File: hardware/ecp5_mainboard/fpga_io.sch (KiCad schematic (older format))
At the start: 75 parts, among them J10 UART, J11 FLASH, J12 JTAG, J5 EXT0, J6 EXT1, J7 EXT2, J8 EXT3, J9 PMOD_01, Q9 BSH111BKR, SW6 SW_Push, U15 ECP5UM5G_85_CABGA756, U26 XL_XO_LVDS, U27 W25Q

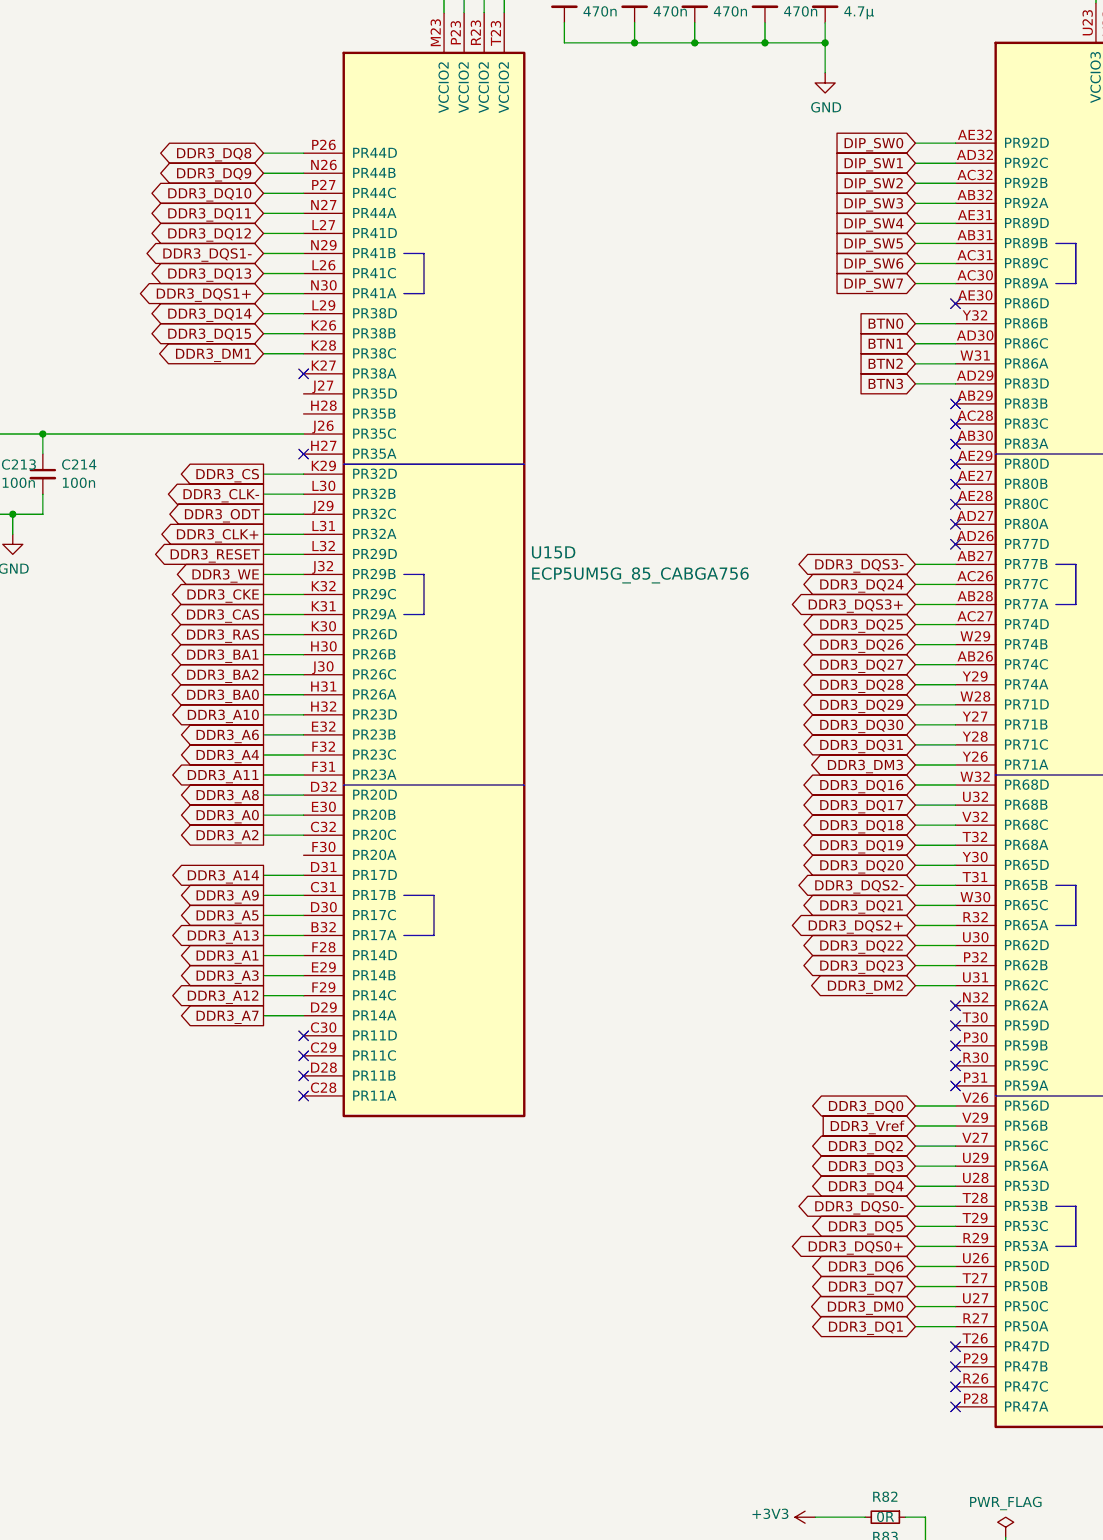
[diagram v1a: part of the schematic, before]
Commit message: hardware/mainboard: Route DDR3 bytes 0 and 1
Signed-off-by: David Shah <dave@ds0.me>
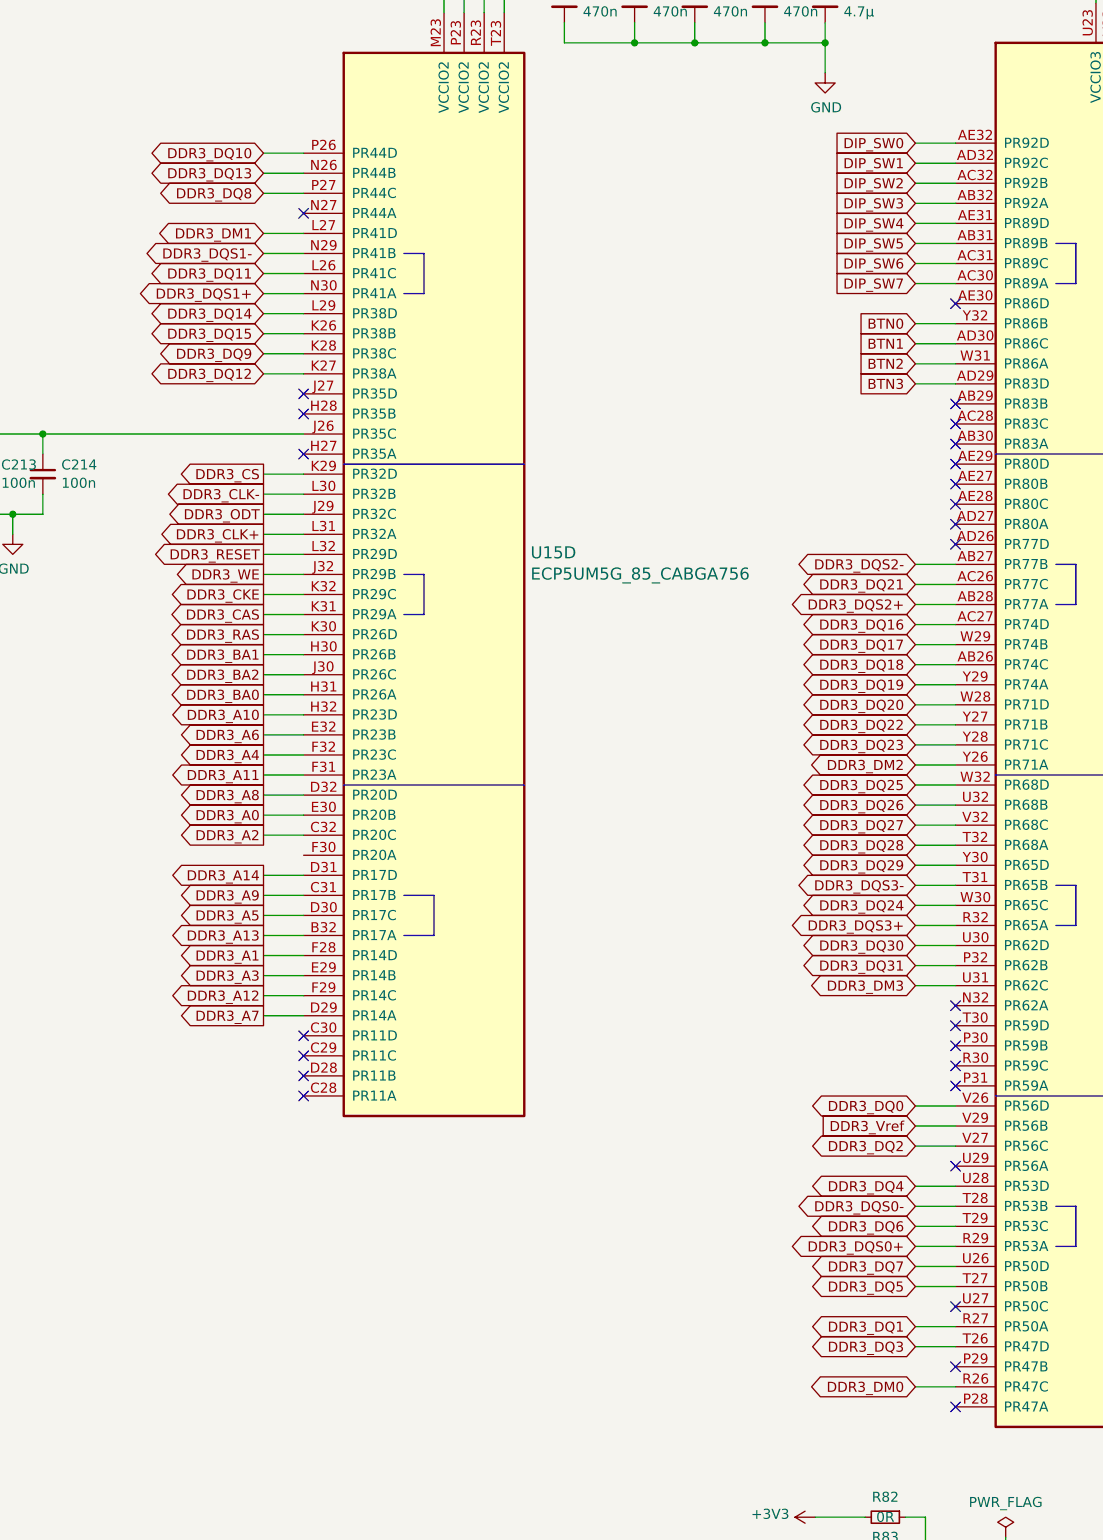
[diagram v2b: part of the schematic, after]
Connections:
- net DDR3_DM0: now also U15.R26 (PR47C); no longer U15.U27 (PR50C)
- net DDR3_DM1: now also U15.L27 (PR41D); no longer U15.K28 (PR38C)
- net DDR3_DM2: now also U15.Y26 (PR71A); no longer U15.U31 (PR62C)
- net DDR3_DM3: now also U15.U31 (PR62C); no longer U15.Y26 (PR71A)
- net DDR3_DQ10: now also U15.P26 (PR44D); no longer U15.P27 (PR44C)
- net DDR3_DQ11: now also U15.L26 (PR41C); no longer U15.N27 (PR44A)
- net DDR3_DQ12: now also U15.K27 (PR38A); no longer U15.L27 (PR41D)
- net DDR3_DQ13: now also U15.N26 (PR44B); no longer U15.L26 (PR41C)
- net DDR3_DQ16: now also U15.AC27 (PR74D); no longer U15.W32 (PR68D)
- net DDR3_DQ17: now also U15.W29 (PR74B); no longer U15.U32 (PR68B)
- net DDR3_DQ18: now also U15.AB26 (PR74C); no longer U15.V32 (PR68C)
- net DDR3_DQ19: now also U15.Y29 (PR74A); no longer U15.T32 (PR68A)
- net DDR3_DQ20: now also U15.W28 (PR71D); no longer U15.Y30 (PR65D)
- net DDR3_DQ21: now also U15.AC26 (PR77C); no longer U15.W30 (PR65C)
- net DDR3_DQ22: now also U15.Y27 (PR71B); no longer U15.U30 (PR62D)
- net DDR3_DQ23: now also U15.Y28 (PR71C); no longer U15.P32 (PR62B)
- net DDR3_DQ24: now also U15.W30 (PR65C); no longer U15.AC26 (PR77C)
- net DDR3_DQ25: now also U15.W32 (PR68D); no longer U15.AC27 (PR74D)
- net DDR3_DQ26: now also U15.U32 (PR68B); no longer U15.W29 (PR74B)
- net DDR3_DQ27: now also U15.V32 (PR68C); no longer U15.AB26 (PR74C)
- net DDR3_DQ28: now also U15.T32 (PR68A); no longer U15.Y29 (PR74A)
- net DDR3_DQ29: now also U15.Y30 (PR65D); no longer U15.W28 (PR71D)
- net DDR3_DQ3: now also U15.T26 (PR47D); no longer U15.U29 (PR56A)
- net DDR3_DQ30: now also U15.U30 (PR62D); no longer U15.Y27 (PR71B)
- net DDR3_DQ31: now also U15.P32 (PR62B); no longer U15.Y28 (PR71C)
- net DDR3_DQ5: now also U15.T27 (PR50B); no longer U15.T29 (PR53C)
- net DDR3_DQ6: now also U15.T29 (PR53C); no longer U15.U26 (PR50D)
- net DDR3_DQ7: now also U15.U26 (PR50D); no longer U15.T27 (PR50B)
- net DDR3_DQ8: now also U15.P27 (PR44C); no longer U15.P26 (PR44D)
- net DDR3_DQ9: now also U15.K28 (PR38C); no longer U15.N26 (PR44B)
- net DDR3_DQS2+: now also U15.AB28 (PR77A); no longer U15.R32 (PR65A)
- net DDR3_DQS2-: now also U15.AB27 (PR77B); no longer U15.T31 (PR65B)
- net DDR3_DQS3+: now also U15.R32 (PR65A); no longer U15.AB28 (PR77A)
- net DDR3_DQS3-: now also U15.T31 (PR65B); no longer U15.AB27 (PR77B)
- no-connect marks 61 -> 63
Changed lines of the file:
@@
 Text GLabel 2150 2450 0    50   BiDi ~ 0
 DDR3_DQS1-
-Text GLabel 2150 1950 0    50   BiDi ~ 0
+Text GLabel 2150 2150 0    50   BiDi ~ 0
 DDR3_DQ8
-Text GLabel 2150 2050 0    50   BiDi ~ 0
+Text GLabel 2150 2950 0    50   BiDi ~ 0
 DDR3_DQ9
-Text GLabel 2150 2150 0    50   BiDi ~ 0
+Text GLabel 2150 1950 0    50   BiDi ~ 0
 DDR3_DQ10
-Text GLabel 2150 2250 0    50   BiDi ~ 0
+Text GLabel 2150 2550 0    50   BiDi ~ 0
 DDR3_DQ11
-Text GLabel 2150 2350 0    50   BiDi ~ 0
+Text GLabel 2150 3050 0    50   BiDi ~ 0
 DDR3_DQ12
-Text GLabel 2150 2550 0    50   BiDi ~ 0
+Text GLabel 2150 2050 0    50   BiDi ~ 0
 DDR3_DQ13
 Text GLabel 2150 2750 0    50   BiDi ~ 0
@@
 Text GLabel 2150 2850 0    50   BiDi ~ 0
 DDR3_DQ15
-Text GLabel 2150 2950 0    50   BiDi ~ 0
+Text GLabel 2150 2350 0    50   BiDi ~ 0
 DDR3_DM1
 Wire Wire Line
-	2150 1950 2350 1950
+	2150 2150 2350 2150
 Wire Wire Line
-	2150 2050 2350 2050
+	2150 2950 2350 2950
 Wire Wire Line
-	2150 2150 2350 2150
+	2150 1950 2350 1950
 Wire Wire Line
-	2150 2250 2350 2250
+	2150 2550 2350 2550
 Wire Wire Line
-	2150 2350 2350 2350
+	2150 3050 2350 3050
 Wire Wire Line
 	2150 2450 2350 2450
 Wire Wire Line
-	2150 2550 2350 2550
+	2150 2050 2350 2050
 Wire Wire Line
 	2150 2650 2350 2650
@@
 	2150 2850 2350 2850
 Wire Wire Line
-	2150 2950 2350 2950
+	2150 2350 2350 2350
 Wire Wire Line
 	15400 1800 14800 1800
@@
 Text Label 14800 2000 0    50   ~ 0
 CLK100+
-Text GLabel 5400 5800 0    50   BiDi ~ 0
+Text GLabel 5400 4200 0    50   BiDi ~ 0
 DDR3_DQS2+
-Text GLabel 5400 5600 0    50   BiDi ~ 0
+Text GLabel 5400 4000 0    50   BiDi ~ 0
 DDR3_DQS2-
-Text GLabel 5400 5100 0    50   BiDi ~ 0
+Text GLabel 5400 4300 0    50   BiDi ~ 0
 DDR3_DQ16
-Text GLabel 5400 5200 0    50   BiDi ~ 0
+Text GLabel 5400 4400 0    50   BiDi ~ 0
 DDR3_DQ17
-Text GLabel 5400 5300 0    50   BiDi ~ 0
+Text GLabel 5400 4500 0    50   BiDi ~ 0
 DDR3_DQ18
-Text GLabel 5400 5400 0    50   BiDi ~ 0
+Text GLabel 5400 4600 0    50   BiDi ~ 0
 DDR3_DQ19
-Text GLabel 5400 5500 0    50   BiDi ~ 0
+Text GLabel 5400 4700 0    50   BiDi ~ 0
 DDR3_DQ20
-Text GLabel 5400 5700 0    50   BiDi ~ 0
+Text GLabel 5400 4100 0    50   BiDi ~ 0
 DDR3_DQ21
-Text GLabel 5400 5900 0    50   BiDi ~ 0
+Text GLabel 5400 4800 0    50   BiDi ~ 0
 DDR3_DQ22
-Text GLabel 5400 6000 0    50   BiDi ~ 0
+Text GLabel 5400 4900 0    50   BiDi ~ 0
 DDR3_DQ23
 Wire Wire Line
-	5400 5100 5600 5100
+	5400 4300 5600 4300
 Wire Wire Line
-	5400 5200 5600 5200
+	5400 4400 5600 4400
 Wire Wire Line
-	5400 5300 5600 5300
+	5400 4500 5600 4500
 Wire Wire Line
-	5400 5400 5600 5400
+	5400 4600 5600 4600
 Wire Wire Line
-	5400 5500 5600 5500
+	5400 4700 5600 4700
 Wire Wire Line
-	5400 5600 5600 5600
+	5400 4000 5600 4000
 Wire Wire Line
-	5400 5700 5600 5700
+	5400 4100 5600 4100
 Wire Wire Line
-	5400 5800 5600 5800
+	5400 4200 5600 4200
 Wire Wire Line
-	5400 5900 5600 5900
+	5400 4800 5600 4800
 Wire Wire Line
-	5400 6000 5600 6000
-Text GLabel 5400 6100 0    50   BiDi ~ 0
+	5400 4900 5600 4900
+Text GLabel 5400 5000 0    50   BiDi ~ 0
 DDR3_DM2
 Wire Wire Line
-	5400 6100 5600 6100
+	5400 5000 5600 5000
 $Comp
 L Device:C_Small C218
@@
 Wire Wire Line
 	5400 6800 5600 6800
-Text GLabel 5400 4200 0    50   BiDi ~ 0
+Text GLabel 5400 5800 0    50   BiDi ~ 0
 DDR3_DQS3+
 Wire Wire Line
-	5400 4200 5600 4200
-Text GLabel 5400 4000 0    50   BiDi ~ 0
+	5400 5800 5600 5800
+Text GLabel 5400 5600 0    50   BiDi ~ 0
 DDR3_DQS3-
 Wire Wire Line
-	5400 4000 5600 4000
+	5400 5600 5600 5600
 Wire Wire Line
-	5600 4100 5400 4100
-Text GLabel 5400 4100 0    50   BiDi ~ 0
+	5600 5700 5400 5700
+Text GLabel 5400 5700 0    50   BiDi ~ 0
 DDR3_DQ24
-Text GLabel 5400 4300 0    50   BiDi ~ 0
+Text GLabel 5400 5100 0    50   BiDi ~ 0
 DDR3_DQ25
-Text GLabel 5400 4400 0    50   BiDi ~ 0
+Text GLabel 5400 5200 0    50   BiDi ~ 0
 DDR3_DQ26
-Text GLabel 5400 4500 0    50   BiDi ~ 0
+Text GLabel 5400 5300 0    50   BiDi ~ 0
 DDR3_DQ27
-Text GLabel 5400 4600 0    50   BiDi ~ 0
+Text GLabel 5400 5400 0    50   BiDi ~ 0
 DDR3_DQ28
-Text GLabel 5400 4700 0    50   BiDi ~ 0
+Text GLabel 5400 5500 0    50   BiDi ~ 0
 DDR3_DQ29
-Text GLabel 5400 4800 0    50   BiDi ~ 0
+Text GLabel 5400 5900 0    50   BiDi ~ 0
 DDR3_DQ30
-Text GLabel 5400 4900 0    50   BiDi ~ 0
+Text GLabel 5400 6000 0    50   BiDi ~ 0
 DDR3_DQ31
 Wire Wire Line
-	5400 4900 5600 4900
+	5400 6000 5600 6000
 Wire Wire Line
-	5600 4800 5400 4800
+	5600 5900 5400 5900
 Wire Wire Line
-	5400 4700 5600 4700
+	5400 5500 5600 5500
 Wire Wire Line
-	5600 4600 5400 4600
+	5600 5400 5400 5400
 Wire Wire Line
-	5400 4500 5600 4500
+	5400 5300 5600 5300
 Wire Wire Line
-	5600 4400 5400 4400
+	5600 5200 5400 5200
 Wire Wire Line
-	5400 4300 5600 4300
+	5400 5100 5600 5100
 Text GLabel 2150 5250 0    50   Output ~ 0
 DDR3_A0
@@
 Text GLabel 2150 3550 0    50   Output ~ 0
 DDR3_CS
-Text GLabel 5400 5000 0    50   BiDi ~ 0
+Text GLabel 5400 6100 0    50   BiDi ~ 0
 DDR3_DM3
 Wire Wire Line
-	5400 5000 5600 5000
+	5400 6100 5600 6100
 Wire Wire Line
 	2150 3950 2350 3950
@@
 Text GLabel 5400 6900 0    50   BiDi ~ 0
 DDR3_DQ2
-Text GLabel 5400 7000 0    50   BiDi ~ 0
+Text GLabel 5400 7900 0    50   BiDi ~ 0
 DDR3_DQ3
 Text GLabel 5400 7100 0    50   BiDi ~ 0
 DDR3_DQ4
-Text GLabel 5400 7300 0    50   BiDi ~ 0
+Text GLabel 5400 7600 0    50   BiDi ~ 0
 DDR3_DQ5
-Text GLabel 5400 7500 0    50   BiDi ~ 0
+Text GLabel 5400 7300 0    50   BiDi ~ 0
 DDR3_DQ6
-Text GLabel 5400 7600 0    50   BiDi ~ 0
+Text GLabel 5400 7500 0    50   BiDi ~ 0
 DDR3_DQ7
-Text GLabel 5400 7700 0    50   BiDi ~ 0
+Text GLabel 5400 8100 0    50   BiDi ~ 0
 DDR3_DM0
 Wire Wire Line
@@
 	5400 6900 5600 6900
 Wire Wire Line
-	5400 7000 5600 7000
+	5400 7900 5600 7900
 Wire Wire Line
 	5400 7100 5600 7100
@@
 	5400 7200 5600 7200
 Wire Wire Line
-	5400 7300 5600 7300
+	5400 7600 5600 7600
 Wire Wire Line
 	5400 7400 5600 7400
 Wire Wire Line
-	5400 7500 5600 7500
+	5400 7300 5600 7300
 Wire Wire Line
-	5400 7600 5600 7600
+	5400 7500 5600 7500
 Wire Wire Line
-	5400 7700 5600 7700
+	5400 8100 5600 8100
 Text GLabel 5400 1900 0    50   Input ~ 0
 DIP_SW0
@@
 NoConn ~ 5600 6400
 NoConn ~ 5600 6500
-NoConn ~ 5600 7900
 NoConn ~ 5600 8000
-NoConn ~ 5600 8100
 NoConn ~ 5600 8200
 NoConn ~ 20650 5400
@@
 Wire Wire Line
 	20300 5700 20150 5700
-NoConn ~ 2350 3050
 Wire Bus Line
 	2550 5100 3450 5100
@@
 NoConn ~ 5600 3900
 NoConn ~ 5600 3800
+NoConn ~ 2350 3150
+NoConn ~ 2350 3250
+NoConn ~ 2350 2250
+NoConn ~ 5600 7700
+NoConn ~ 5600 7000
 $EndSCHEMATC
